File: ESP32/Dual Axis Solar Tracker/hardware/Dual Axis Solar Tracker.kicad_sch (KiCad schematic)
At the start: 0 parts

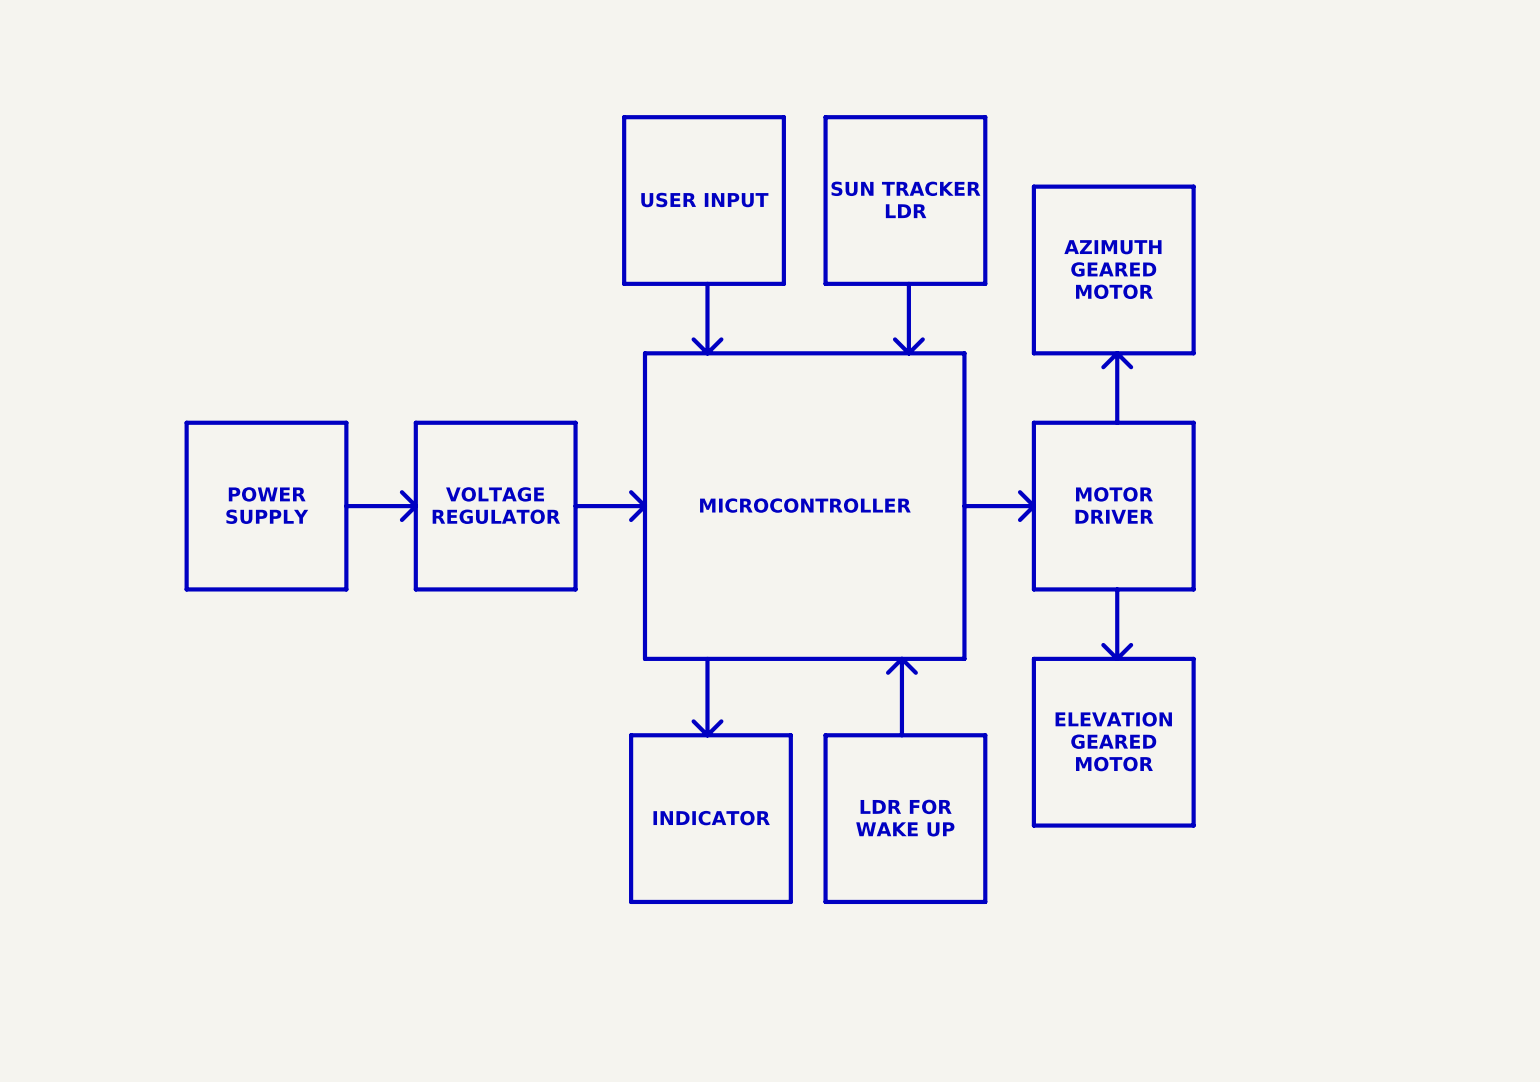
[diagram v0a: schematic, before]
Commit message: Done with schematic
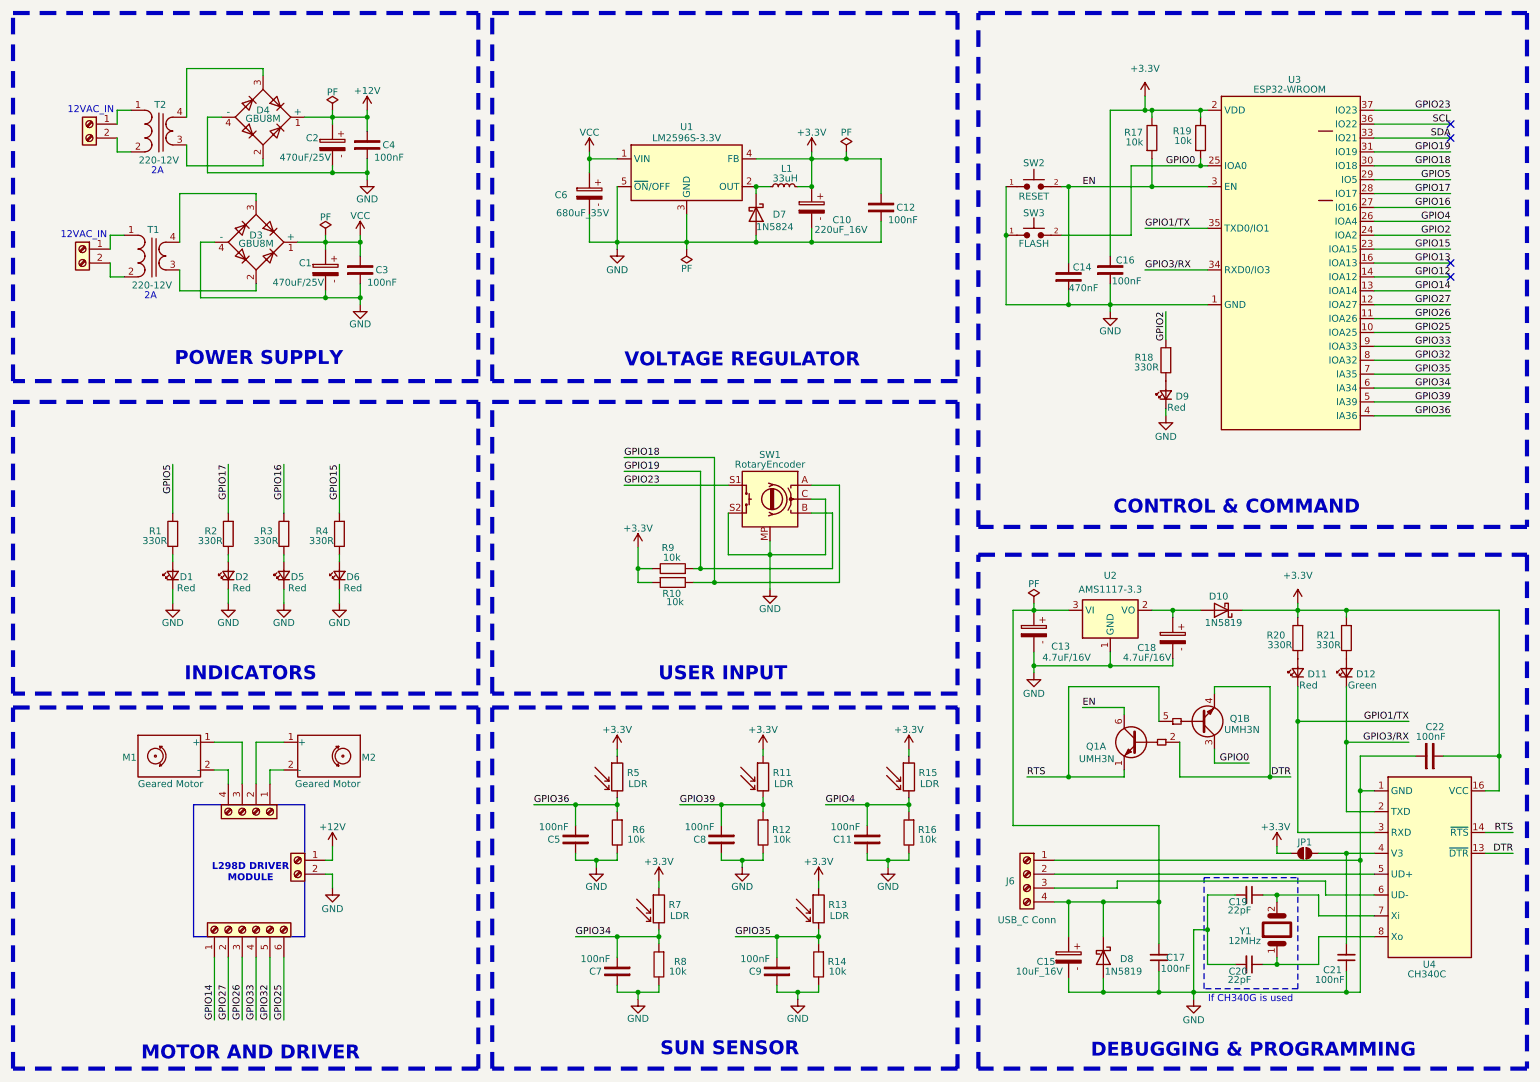
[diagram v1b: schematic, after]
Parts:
- added C1, C2: 470uF/25V, Capacitor_SMD:CP_Elec_10x12.5, symbol PCM_SL_Capacitors:4.7uF_16V
- added C10: 220uF_16V, Capacitor_SMD:CP_Elec_10x12.5, symbol PCM_SL_Capacitors:470uF_35V
- added C11, C12, C16, C22, C3, C4, C5, C7, C8, C9: 100nF, Capacitor_SMD:C_0805_2012Metric_Pad1.18x1.45mm_HandSolder, symbol PCM_SL_Capacitors:104_Ceramic
- added C13, C18: 4.7uF/16V, Capacitor_Tantalum_SMD:CP_EIA-3528-21_Kemet-B_HandSolder, symbol PCM_SL_Capacitors:4.7uF_16V
- added C14: 470nF, Capacitor_SMD:C_0805_2012Metric_Pad1.18x1.45mm_HandSolder, symbol PCM_SL_Capacitors:104_Ceramic
- added C15: 10uF_16V, Capacitor_THT:CP_Radial_D5.0mm_P2.00mm, symbol PCM_SL_Capacitors:10uF_16V
- added C17, C21: 100nF, Capacitor_SMD:C_0805_2012Metric_Pad1.18x1.45mm_HandSolder, symbol Device:C_Small
- added C19, C20: 22pF, Capacitor_SMD:C_0805_2012Metric_Pad1.18x1.45mm_HandSolder, symbol Device:C_Small
- added C6: 680uF_35V, Capacitor_SMD:CP_Elec_10x12.5, symbol PCM_SL_Capacitors:470uF_35V
- added D1, D11, D2, D5, D6, D9: Red, LED_THT:LED_D3.0mm, symbol SparkFun-LED:LED_Red_0603
- added D10: 1N5819, Diode_SMD:D_SMA, symbol Diode:1N5819
- added D12: Green, LED_THT:LED_D3.0mm, symbol SparkFun-LED:LED_Red_0603
- added D3, D4: GBU8M, Diode_THT:Diode_Bridge_Vishay_GBU, symbol Diode_Bridge:GBU8M
- added D7: 1N5824, Diode_SMD:D_SMA, symbol Diode:1N5822
- added D8: 1N5819, Diode_THT:D_DO-41_SOD81_P10.16mm_Horizontal, symbol Diode:1N5819
- added J1, J2: 12VAC, PCM_SparkFun-Connector:ScrewTerminal_1x02_P3.5mm_Horizontal_Black, symbol Connector:Screw_Terminal_01x02
- added J3: SIGNAL, Connector_PinHeader_2.54mm:PinHeader_1x06_P2.54mm_Vertical, symbol Connector:Screw_Terminal_01x06
- added J4: MOTOR, PCM_SparkFun-Connector:ScrewTerminal_1x04_P3.5mm_Locking, symbol Connector:Screw_Terminal_01x04
- added J5: 12V_IN, PCM_SparkFun-Connector:ScrewTerminal_1x02_P3.5mm_Horizontal_Black, symbol Connector:Screw_Terminal_01x02
- added J6: USB_C Conn, Connector_PinHeader_2.54mm:PinHeader_1x04_P2.54mm_Vertical, symbol Connector:Screw_Terminal_01x04
- added JP1: ~, Jumper:SolderJumper-2_P1.3mm_Open_Pad1.0x1.5mm, symbol SparkFun-Jumper:SolderJumper_2_Open
- added L1: 33uH, Inductor_SMD:L_12x12mm_H6mm, symbol Device:L_Small
- added M1, M2: Geared Motor, symbol Motor:Motor_Servo
- added Q1: UMH3N, Package_TO_SOT_SMD:SOT-363_SC-70-6, symbol Transistor_BJT:UMH3N
- added R1, R18, R2, R20, R21, R3, R4: 330R, Resistor_SMD:R_0805_2012Metric, symbol PCM_SL_Resistors:1M
- added R10, R17, R19, R9: 10k, Resistor_SMD:R_0805_2012Metric, symbol PCM_SL_Resistors:10k
- added R11, R13, R15, R5, R7: LDR, OptoDevice:R_LDR_5.1x4.3mm_P3.4mm_Vertical, symbol Sensor_Optical:LDR07
- added R12, R14, R16, R6, R8: 10k, Resistor_SMD:R_0805_2012Metric, symbol PCM_SL_Resistors:1M
- added SW1: RotaryEncoder, symbol Device:RotaryEncoder_Switch_MP
- added SW2: RESET, Button_Switch_SMD:SW_SPST_CK_KXT3, symbol PCM_SL_Devices:Push_Button
- added SW3: FLASH, Button_Switch_SMD:SW_SPST_CK_KXT3, symbol PCM_SL_Devices:Push_Button
- added T1, T2: 220-12V, symbol Device:Transformer_1P_1S
- added U1: LM2596S-3.3V, Package_TO_SOT_SMD:TO-263-5_TabPin6, symbol Regulator_Switching:LM2596S-3.3
- added U2: AMS1117-3.3, Package_TO_SOT_SMD:SOT-223-3_TabPin2, symbol Regulator_Linear:AMS1117-3.3
- added U3: ESP32-WROOM, RF_Module:ESP32-WROOM-32U, symbol SparkFun-RF:ESP32-WROOM
- added U4: CH340C, Package_SO:SOIC-16_3.9x9.9mm_P1.27mm, symbol Interface_USB:CH340C
- added Y1: 12MHz, Crystal:Crystal_HC49-4H_Vertical, symbol PCM_SL_Devices:Crystal_16MHz
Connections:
- new net: D11.2 (A), R20.2
- new net: J2.1 (Pin_1), T2.1 (AA)
- new net: J2.2 (Pin_2), T2.2 (AB)
- new net: D1.2 (A), R1.2
- new net: D6.2 (A), R4.2
- new net: C13.1, C15.1, C17.2, D8.1 (K), J6.4 (Pin_4), U2.3 (VI)
- new net: J6.2 (Pin_2), U4.5 (UD+)
- new net: J6.3 (Pin_3), U4.6 (UD-)
- new net: D9.2 (A), R18.2
- new net: C18.1, D10.2 (A), U2.2 (VO)
- new net: D12.2 (A), R21.2
- new net: D3.2, T1.3 (SA)
- new net: D3.3, T1.4 (SB)
- new net: D7.1 (K), L1.1, U1.2 (OUT)
- new net: D4.2, T2.3 (SA)
- new net: D4.3, T2.4 (SB)
- new net: J4.3 (Pin_3), M1.1 (+)
- new net: J4.4 (Pin_4), M1.2 (-)
- new net: J4.2 (Pin_2), M2.1 (+)
- new net: J4.1 (Pin_1), M2.2 (-)
- new net: C21.2, JP1.1 (A), U4.4 (V3)
- new net: C19.1, U4.7 (Xi), Y1.2
- new net: C20.1, U4.8 (Xo), Y1.1
- new net: D2.2 (A), R2.2
- new net: D5.2 (A), R3.2
- new net: J1.1 (Pin_1), T1.1 (AA)
- new net: J1.2 (Pin_2), T1.2 (AB)
- new net +12V: C2.1, C4.2, D4.1 (+), J5.1 (Pin_1)
- new net +3.3V: C10.1, C12.2, C16.2, C22.1, D10.1 (K), JP1.2 (B), L1.2, R10.1, R11.1, R13.1, R15.1, R17.2, R19.2, R20.1, R21.1, R5.1, R7.1, R9.2, U1.4 (FB), U3.2 (VDD), U4.16 (VCC)
- new net DTR: Q1.2 (B1), Q1.4 (E2), U4.13 (~{DTR})
- new net EN: C14.2, Q1.6 (C1), R17.1, SW2.2, U3.3 (EN)
- new net GND: C1.2, C10.2, C11.2, C12.1, C13.2, C14.1, C15.2, C16.1, C17.1, C18.2, C19.2, C2.2, C20.2, C21.1, C22.2, C3.1, C4.1, C5.2, C6.2, C7.2, C8.2, C9.2, D1.1 (K), D2.1 (K), D3.4 (-), D4.4 (-), D5.1 (K), D6.1 (K), D7.2 (A), D8.2 (A), D9.1 (K), J5.2 (Pin_2), J6.1 (Pin_1), R12.2, R14.2, R16.2, R6.2, R8.2, SW1.C, SW1.MP, SW1.S2, SW2.1, SW3.1, U1.3 (GND), U1.5 (~{ON}/OFF), U1.6 (GND), U2.1 (GND), U3.1 (GND), U3.15 (GND), U3.38 (GND), U3.39 (GND), U4.1 (GND)
- new net GPIO0: Q1.3 (C2), R19.1, SW3.2, U3.25 (IOA0)
- new net GPIO12: U3.14 (IOA12)
- new net GPIO13: U3.16 (IOA13)
- new net GPIO14: J3.1 (Pin_1), U3.13 (IOA14)
- new net GPIO15: R4.1, U3.23 (IOA15)
- new net GPIO16: R3.1, U3.27 (IO16)
- new net GPIO17: R2.1, U3.28 (IO17)
- new net GPIO18: R10.2, SW1.A, U3.30 (IO18)
- new net GPIO19: R9.1, SW1.B, U3.31 (IO19)
- new net GPIO1/TX: D11.1 (K), U3.35 (TXD0/IO1), U4.3 (RXD)
- new net GPIO2: R18.1, U3.24 (IOA2)
- new net GPIO23: SW1.S1, U3.37 (IO23)
- new net GPIO25: J3.6 (Pin_6), U3.10 (IOA25)
- new net GPIO26: J3.3 (Pin_3), U3.11 (IOA26)
- new net GPIO27: J3.2 (Pin_2), U3.12 (IOA27)
- new net GPIO32: J3.5 (Pin_5), U3.8 (IOA32)
- new net GPIO33: J3.4 (Pin_4), U3.9 (IOA33)
- new net GPIO34: C7.1, R7.2, R8.1, U3.6 (IA34)
- new net GPIO35: C9.1, R13.2, R14.1, U3.7 (IA35)
- new net GPIO36: C5.1, R5.2, R6.1, U3.4 (IA36)
- new net GPIO39: C8.1, R11.2, R12.1, U3.5 (IA39)
- new net GPIO3/RX: D12.1 (K), U3.34 (RXD0/IO3), U4.2 (TXD)
- new net GPIO4: C11.1, R15.2, R16.1, U3.26 (IOA4)
- new net GPIO5: R1.1, U3.29 (IO5)
- new net RTS: Q1.1 (E1), Q1.5 (B2), U4.14 (~{RTS})
- new net SCL: U3.36 (IO22)
- new net SDA: U3.33 (IO21)
- new net VCC: C1.1, C3.2, C6.1, D3.1 (+), U1.1 (VIN)
- no-connect marks 0 -> 4
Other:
- note added: "12VAC_IN"
- note added: "2A"
- note added: "CONTROL & COMMAND"
- note added: "DEBUGGING & PROGRAMMING"
- note added: "INDICATORS"
- note added: "If CH340G is used"
- note added: "L298D DRIVER MODULE"
- note added: "MOTOR AND DRIVER"
- note added: "POWER SUPPLY"
- note added: "SUN SENSOR"
- note added: "USER INPUT"
- note added: "VOLTAGE REGULATOR"
